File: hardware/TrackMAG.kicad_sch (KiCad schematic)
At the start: 57 parts, among them J1 USB_C_Socket_USB2.0, J2 Conn_Debug, SW1 SW_RESET, SW2 SW_BOOT, SW3 SW_CALIBRATE, U1 LSM6DS3TR-C, U2 USBLC6-2P6, U3 STM32F103C8T6, U4 LIS2MDL, U5 AMS1117-3.3, Y1 16MHz

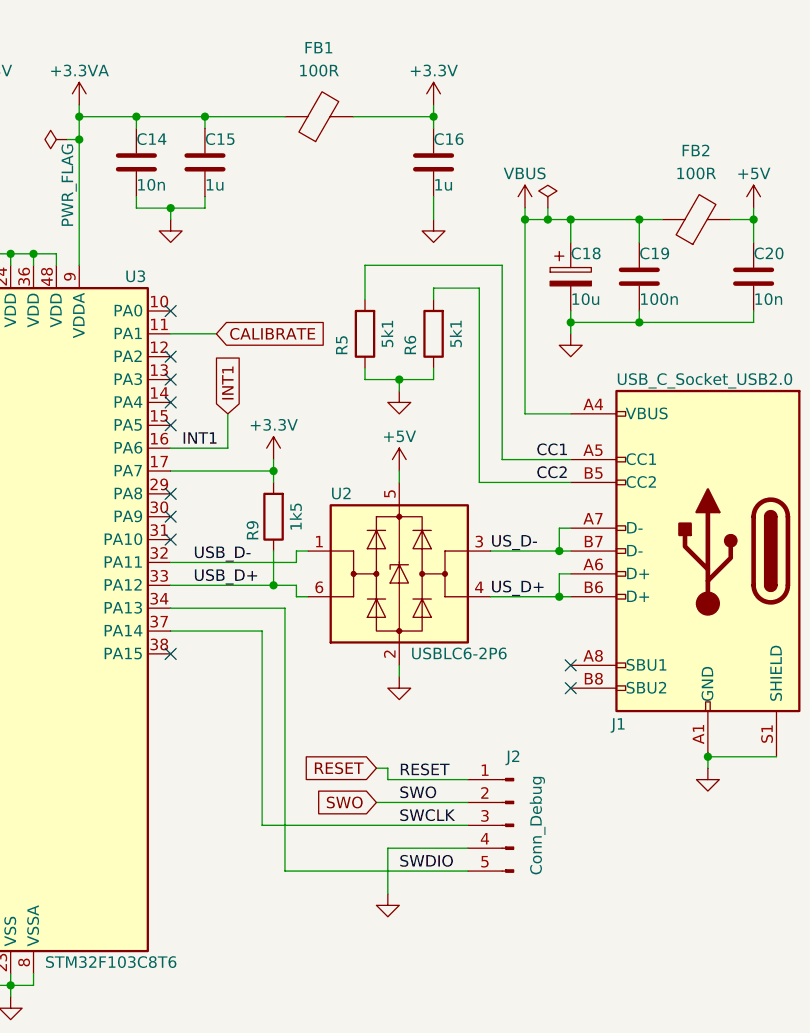
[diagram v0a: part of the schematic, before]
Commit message: Fix various problems, cleanup after review
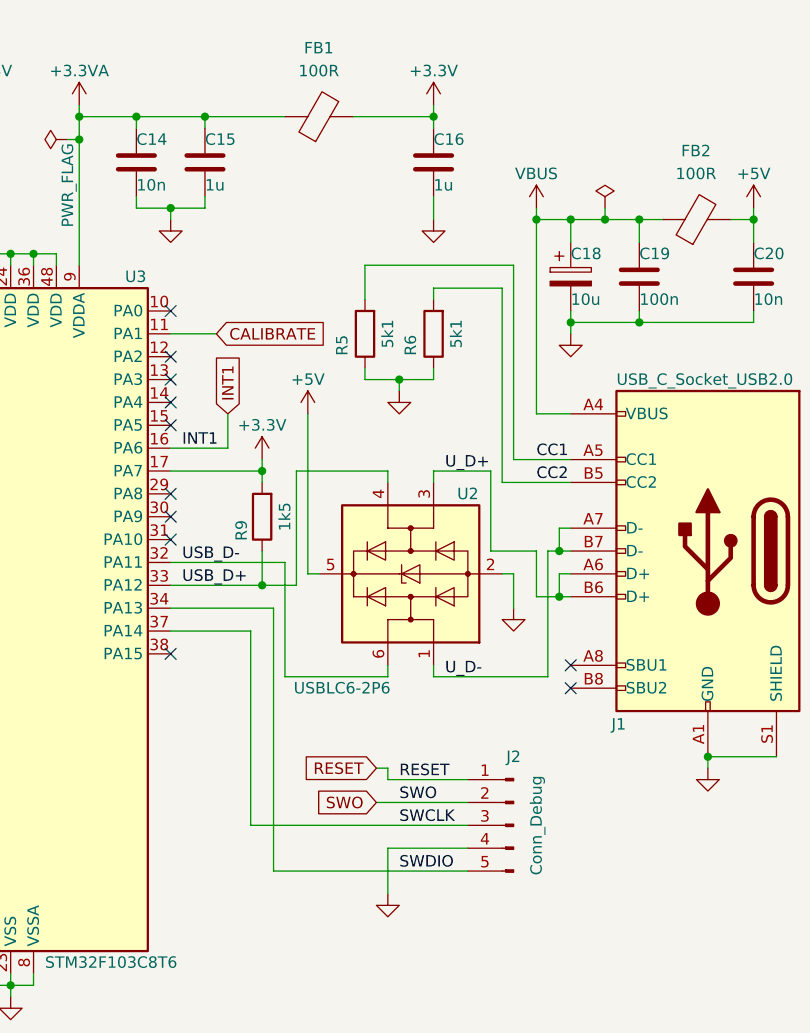
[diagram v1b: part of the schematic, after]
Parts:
- removed U2: USBLC6-2P6, TrackMAG:SOT-666, symbol USBLC6-2P:USBLC6-2P6
- added U2: USBLC6-2P6, TrackMAG:SOT-666, symbol Power_Protection:USBLC6-2P6
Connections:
- net +5V: now also U2.5 (VBUS)
- net GND: now also U2.2 (GND)
- net USB_D+: now also U2.4 (I/O2)
- net USB_D-: now also U2.6 (I/O1)
- net US_D+ renamed U_D+
- net U_D+: now also U2.3 (I/O2)
- net US_D- renamed U_D-
- net U_D-: now also U2.1 (I/O1)
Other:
- moved on the sheet: R9
